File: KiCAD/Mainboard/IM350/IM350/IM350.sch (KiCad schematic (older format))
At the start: 11 parts, among them J1 USB_B_Micro_Power, J2 Conn_02x03_Odd_Even, Q1 BC547, SW1 SW_Push, U1 AMS1117-3.3, U2 ESP-12F

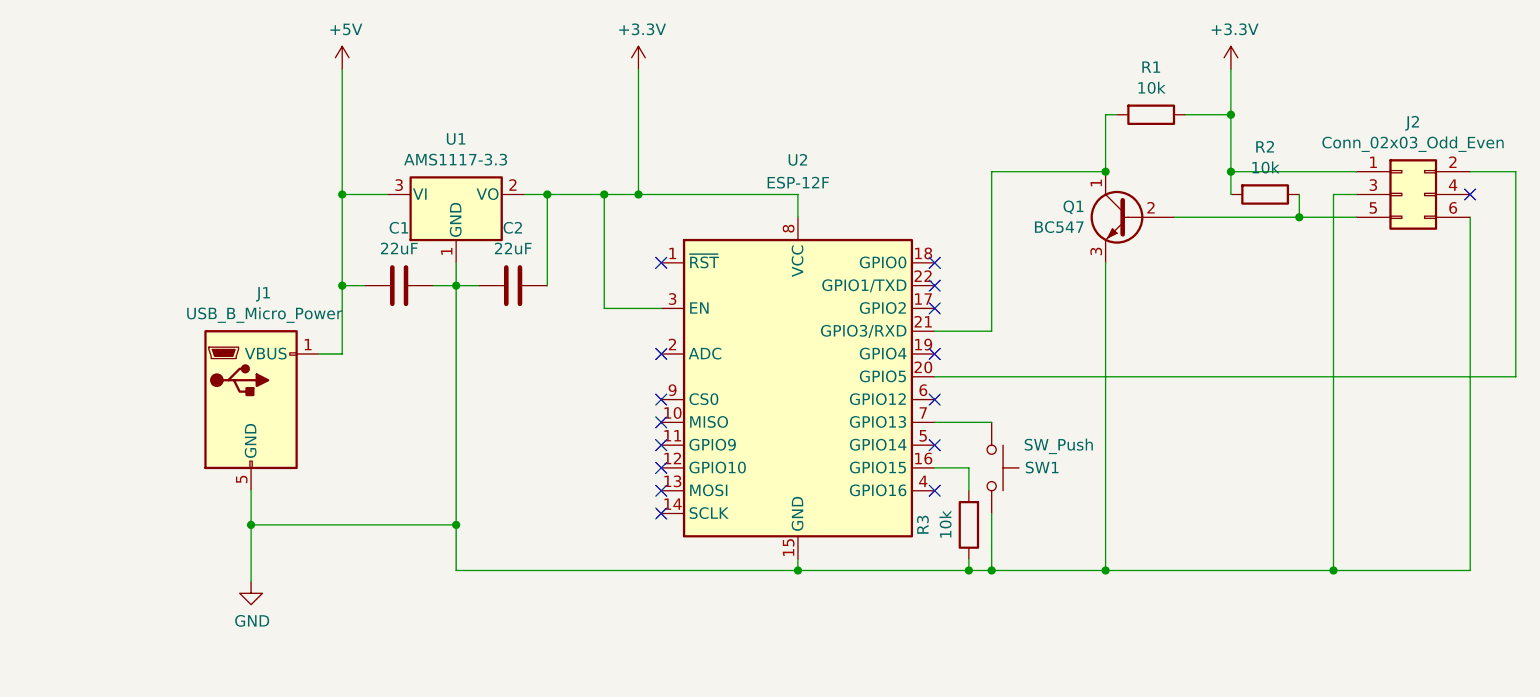
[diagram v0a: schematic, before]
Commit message: Update
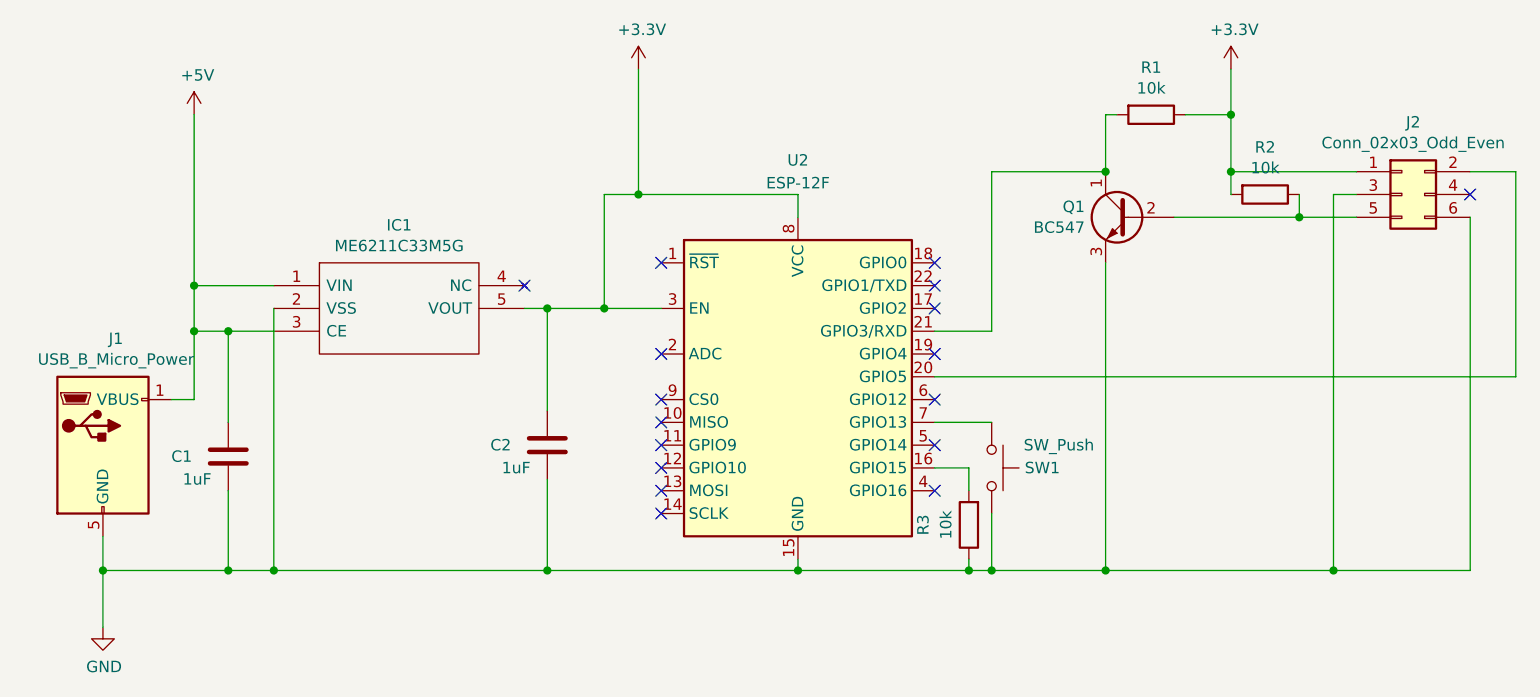
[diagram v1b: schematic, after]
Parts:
- removed U1: AMS1117-3.3, Package_TO_SOT_SMD:SOT-223-3_TabPin2, symbol Regulator_Linear:AMS1117-3.3
- added IC1: ME6211C33M5G, ErichCollection:SOT95P282X145-5N, symbol ME6211C33M5G:ME6211C33M5G
- C1, C2: value 22uF -> 1uF; footprint Capacitor_SMD:C_1206_3216Metric_Pad1.33x1.80mm_HandSolder -> Capacitor_SMD:C_0805_2012Metric_Pad1.18x1.45mm_HandSolder
- J2: footprint Connector_PinHeader_2.54mm:PinHeader_2x03_P2.54mm_Horizontal -> Connector_PinHeader_2.54mm:PinHeader_2x03_P2.54mm_Vertical
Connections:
- net +3V3: now also IC1.5 (VOUT)
- net +5V: now also C1.1, IC1.1 (VIN), IC1.3 (CE); no longer C1.2
- net GND: now also C1.2, IC1.2 (VSS); no longer C1.1
- no-connect marks 16 -> 17
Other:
- moved on the sheet: J1
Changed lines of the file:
@@
 $EndComp
-$Comp
-L Regulator_Linear:AMS1117-3.3 U1
-U 1 1 6053B5FB
-P 2850 2000
-F 0 "U1" H 2850 2242 50  0000 C CNN
-F 1 "AMS1117-3.3" H 2850 2151 50  0000 C CNN
-F 2 "Package_TO_SOT_SMD:SOT-223-3_TabPin2" H 2850 2200 50  0001 C CNN
-F 3 "http://www.advanced-monolithic.com/pdf/ds1117.pdf" H 2950 1750 50  0001 C CNN
-F 4 "C6186" H 2850 2000 50  0001 C CNN "LCSC"
-	1    2850 2000
-	1    0    0    -1
-$EndComp
-Wire Wire Line
-	2350 2000 2550 2000
 $Comp
 L power:GND #PWR01
 U 1 1 6053D4D6
-P 1950 3700
-F 0 "#PWR01" H 1950 3450 50  0001 C CNN
-F 1 "GND" H 1955 3527 50  0000 C CNN
-F 2 "" H 1950 3700 50  0001 C CNN
-F 3 "" H 1950 3700 50  0001 C CNN
-	1    1950 3700
-	1    0    0    -1
-$EndComp
-Wire Wire Line
-	1950 3300 1950 3450
-Wire Wire Line
-	2850 2300 2850 2400
-Wire Wire Line
-	2850 3450 1950 3450
-Connection ~ 1950 3450
-Wire Wire Line
-	1950 3450 1950 3700
-Wire Wire Line
-	2850 3450 2850 3650
-Connection ~ 2850 3450
-Wire Wire Line
-	2450 2400 2350 2400
-Wire Wire Line
-	2350 2400 2350 2000
-Wire Wire Line
-	2750 2400 2850 2400
-Connection ~ 2850 2400
-Wire Wire Line
-	2850 2400 2850 3450
+P 1300 3900
+F 0 "#PWR01" H 1300 3650 50  0001 C CNN
+F 1 "GND" H 1305 3727 50  0000 C CNN
+F 2 "" H 1300 3900 50  0001 C CNN
+F 3 "" H 1300 3900 50  0001 C CNN
+	1    1300 3900
+	1    0    0    -1
+$EndComp
+Wire Wire Line
+	1300 3500 1300 3650
+Connection ~ 1300 3650
+Wire Wire Line
+	1300 3650 1300 3900
 Wire Wire Line
 	4350 3650 4350 3600
@@
 	4350 2000 4350 2100
 Wire Wire Line
-	3150 2000 3250 2000
-Wire Wire Line
-	3250 2400 3250 2000
-Connection ~ 3250 2000
-Wire Wire Line
-	2950 2400 2850 2400
-Wire Wire Line
 	3500 2000 3500 2500
 Wire Wire Line
 	3500 2500 3750 2500
-Connection ~ 3500 2000
 Wire Wire Line
 	3500 2000 3650 2000
@@
 L power:+5V #PWR02
 U 1 1 6054595C
-P 2350 1450
-F 0 "#PWR02" H 2350 1300 50  0001 C CNN
-F 1 "+5V" H 2365 1623 50  0000 C CNN
-F 2 "" H 2350 1450 50  0001 C CNN
-F 3 "" H 2350 1450 50  0001 C CNN
-	1    2350 1450
-	1    0    0    -1
-$EndComp
-Connection ~ 2350 2000
+P 1700 1650
+F 0 "#PWR02" H 1700 1500 50  0001 C CNN
+F 1 "+5V" H 1715 1823 50  0000 C CNN
+F 2 "" H 1700 1650 50  0001 C CNN
+F 3 "" H 1700 1650 50  0001 C CNN
+	1    1700 1650
+	1    0    0    -1
+$EndComp
 Wire Wire Line
 	5700 2300 5700 3650
@@
 F 0 "J2" H 7050 2317 50  0000 C CNN
 F 1 "Conn_02x03_Odd_Even" H 7050 2226 50  0000 C CNN
-F 2 "Connector_PinHeader_2.54mm:PinHeader_2x03_P2.54mm_Horizontal" H 7000 2000 50  0001 C CNN
+F 2 "Connector_PinHeader_2.54mm:PinHeader_2x03_P2.54mm_Vertical" H 7000 2000 50  0001 C CNN
 F 3 "~" H 7000 2000 50  0001 C CNN
 	1    7000 2000
@@
 	1    0    0    -1
 $EndComp
-Wire Wire Line
-	2350 2000 2350 1450
 Wire Wire Line
 	3650 1450 3650 2000
@@
 NoConn ~ 7300 2000
 Wire Wire Line
-	2350 2400 2350 2700
-Wire Wire Line
-	2350 2700 2250 2700
-Connection ~ 2350 2400
+	1700 2900 1600 2900
 Wire Wire Line
 	4350 3650 5100 3650
@@
 Connection ~ 5700 1900
 $Comp
-L Device:C C1
-U 1 1 605964A3
-P 2600 2400
-F 0 "C1" V 2348 2400 50  0000 C CNN
-F 1 "22uF" V 2439 2400 50  0000 C CNN
-F 2 "Capacitor_SMD:C_1206_3216Metric_Pad1.33x1.80mm_HandSolder" H 2638 2250 50  0001 C CNN
-F 3 "~" H 2600 2400 50  0001 C CNN
-	1    2600 2400
-	0    1    1    0
-$EndComp
-$Comp
-L Device:C C2
-U 1 1 60596E7D
-P 3100 2400
-F 0 "C2" V 2848 2400 50  0000 C CNN
-F 1 "22uF" V 2939 2400 50  0000 C CNN
-F 2 "Capacitor_SMD:C_1206_3216Metric_Pad1.33x1.80mm_HandSolder" H 3138 2250 50  0001 C CNN
-F 3 "~" H 3100 2400 50  0001 C CNN
-	1    3100 2400
-	0    1    1    0
-$EndComp
-Wire Wire Line
-	3250 2000 3500 2000
-Wire Wire Line
-	2850 3650 4350 3650
-$Comp
 L Device:R R3
 U 1 1 60596A0F
@@
 L Erich:USB_B_Micro_Power J1
 U 1 1 605D392E
-P 1950 2900
-F 0 "J1" H 2007 3367 50  0000 C CNN
-F 1 "USB_B_Micro_Power" H 2007 3276 50  0000 C CNN
-F 2 "SHRDZM:USB_Micro-B_Power" H 2100 2850 50  0001 C CNN
-F 3 "~" H 2100 2850 50  0001 C CNN
-	1    1950 2900
-	1    0    0    -1
-$EndComp
+P 1300 3100
+F 0 "J1" H 1357 3567 50  0000 C CNN
+F 1 "USB_B_Micro_Power" H 1357 3476 50  0000 C CNN
+F 2 "SHRDZM:USB_Micro-B_Power" H 1450 3050 50  0001 C CNN
+F 3 "~" H 1450 3050 50  0001 C CNN
+	1    1300 3100
+	1    0    0    -1
+$EndComp
+$Comp
+L ME6211C33M5G:ME6211C33M5G IC1
+U 1 1 6059B393
+P 2050 2400
+F 0 "IC1" H 2600 2665 50  0000 C CNN
+F 1 "ME6211C33M5G" H 2600 2574 50  0000 C CNN
+F 2 "ErichCollection:SOT95P282X145-5N" H 3000 2500 50  0001 L CNN
+F 3 "http://xinhuidianzi.com.cn/UploadSysFiles/files/LDO-series/ME6211-Series_E15.0.pdf" H 3000 2400 50  0001 L CNN
+F 4 "High Speed LDO Regulators, High PSRR, Low noise, ME6211 Series" H 3000 2300 50  0001 L CNN "Description"
+F 5 "1.45" H 3000 2200 50  0001 L CNN "Height"
+F 6 "Microne" H 3000 2100 50  0001 L CNN "Manufacturer_Name"
+F 7 "ME6211C33M5G" H 3000 2000 50  0001 L CNN "Manufacturer_Part_Number"
+F 8 "" H 3000 1900 50  0001 L CNN "Mouser Part Number"
+F 9 "" H 3000 1800 50  0001 L CNN "Mouser Price/Stock"
+F 10 "" H 3000 1700 50  0001 L CNN "Arrow Part Number"
+F 11 "" H 3000 1600 50  0001 L CNN "Arrow Price/Stock"
+	1    2050 2400
+	1    0    0    -1
+$EndComp
+Wire Wire Line
+	1700 1650 1700 2400
+Wire Wire Line
+	2050 2400 1700 2400
+Connection ~ 1700 2400
+Wire Wire Line
+	1700 2400 1700 2600
+Connection ~ 1700 2600
+Wire Wire Line
+	1700 2600 1700 2900
+$Comp
+L Device:C C1
+U 1 1 605A350B
+P 1850 3150
+F 0 "C1" H 1600 3150 50  0000 L CNN
+F 1 "1uF" H 1650 3050 50  0000 L CNN
+F 2 "Capacitor_SMD:C_0805_2012Metric_Pad1.18x1.45mm_HandSolder" H 1888 3000 50  0001 C CNN
+F 3 "~" H 1850 3150 50  0001 C CNN
+	1    1850 3150
+	1    0    0    -1
+$EndComp
+Wire Wire Line
+	1700 2600 1850 2600
+Wire Wire Line
+	1300 3650 1850 3650
+Wire Wire Line
+	1850 2600 1850 3000
+Connection ~ 1850 2600
+Wire Wire Line
+	1850 2600 2050 2600
+Wire Wire Line
+	1850 3300 1850 3650
+Connection ~ 1850 3650
+Wire Wire Line
+	1850 3650 2050 3650
+Connection ~ 2050 3650
+Wire Wire Line
+	2050 3650 3250 3650
+Wire Wire Line
+	3150 2500 3250 2500
+Connection ~ 3500 2500
+$Comp
+L Device:C C2
+U 1 1 605A8CD5
+P 3250 3100
+F 0 "C2" H 3000 3100 50  0000 L CNN
+F 1 "1uF" H 3050 3000 50  0000 L CNN
+F 2 "Capacitor_SMD:C_0805_2012Metric_Pad1.18x1.45mm_HandSolder" H 3288 2950 50  0001 C CNN
+F 3 "~" H 3250 3100 50  0001 C CNN
+	1    3250 3100
+	1    0    0    -1
+$EndComp
+Wire Wire Line
+	3250 2950 3250 2500
+Connection ~ 3250 2500
+Wire Wire Line
+	3250 3250 3250 3650
+Connection ~ 3250 3650
+Wire Wire Line
+	3250 3650 4350 3650
+NoConn ~ 3150 2400
+Wire Wire Line
+	2050 2500 2050 3650
+Wire Wire Line
+	3250 2500 3500 2500
 $EndSCHEMATC
